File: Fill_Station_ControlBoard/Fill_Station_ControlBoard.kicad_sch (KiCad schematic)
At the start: 0 parts

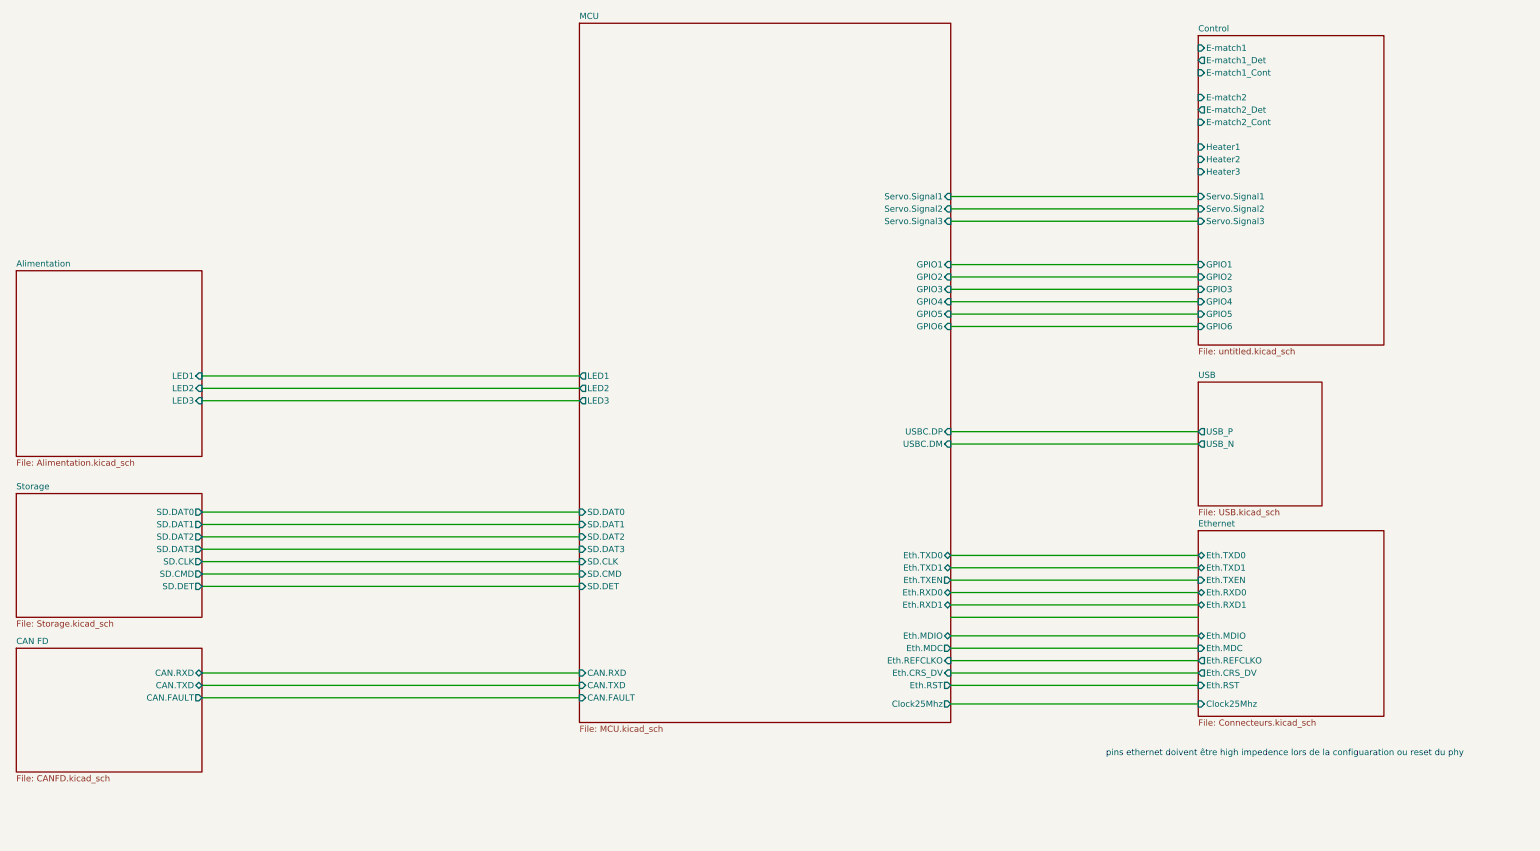
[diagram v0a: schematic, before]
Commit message: PCB fait
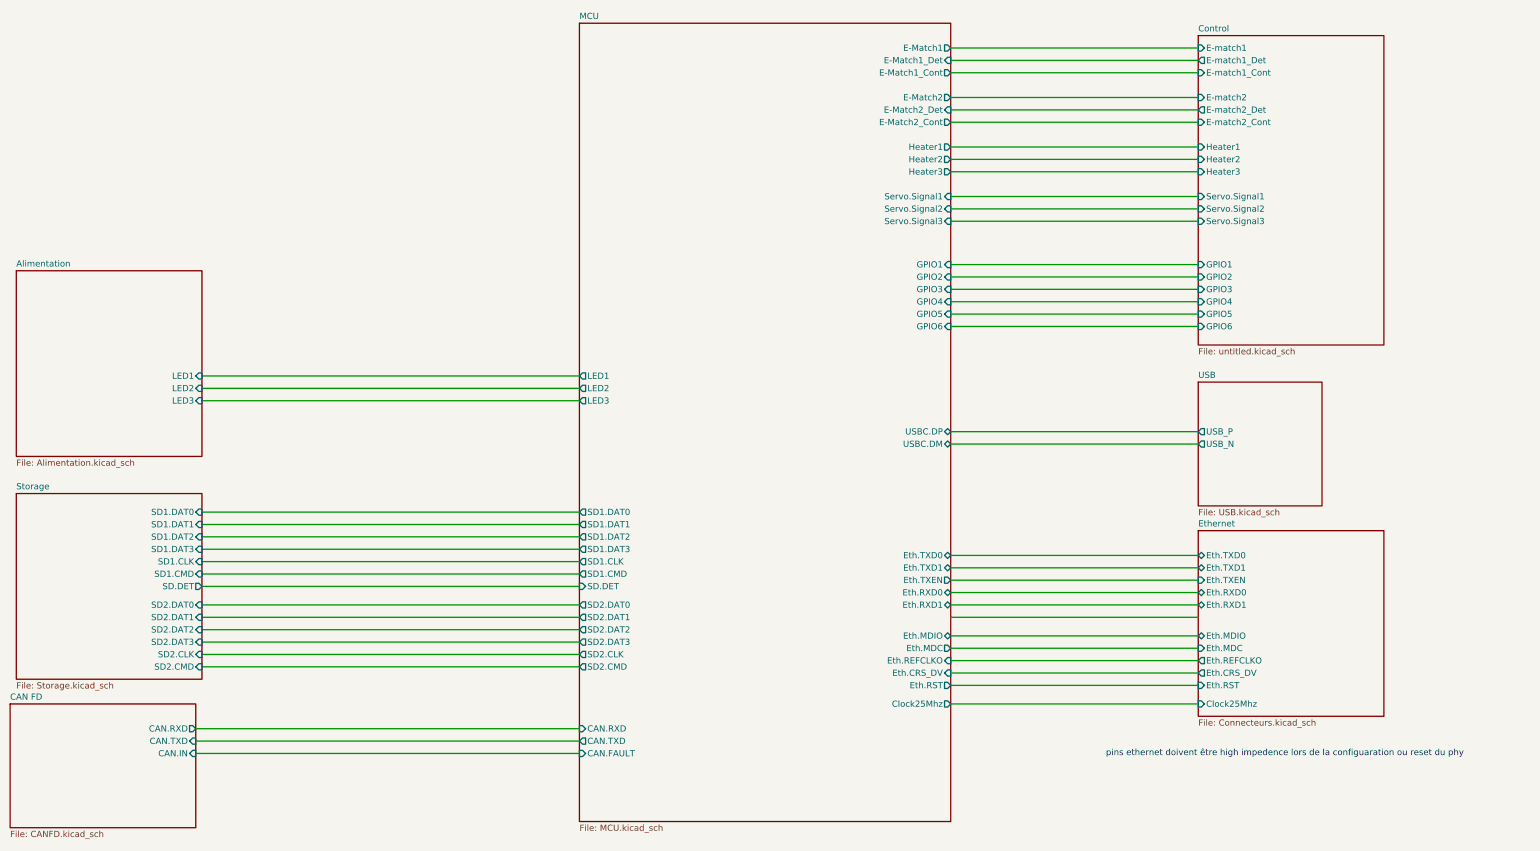
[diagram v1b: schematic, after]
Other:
- sheet CAN FD ports: added CAN.IN; removed CAN.FAULT
- sheet MCU ports: added E-Match1, E-Match1_Cont, E-Match1_Det, E-Match2, E-Match2_Cont, E-Match2_Det, Heater1, Heater2, Heater3, SD1.CLK, SD1.CMD, SD1.DAT0, SD1.DAT1, SD1.DAT2, SD1.DAT3, SD2.CLK, SD2.CMD, SD2.DAT0, SD2.DAT1, SD2.DAT2, SD2.DAT3; removed SD.CLK, SD.CMD, SD.DAT0, SD.DAT1, SD.DAT2, SD.DAT3
- sheet Storage ports: added SD1.CLK, SD1.CMD, SD1.DAT0, SD1.DAT1, SD1.DAT2, SD1.DAT3, SD2.CLK, SD2.CMD, SD2.DAT0, SD2.DAT1, SD2.DAT2, SD2.DAT3; removed SD.CLK, SD.CMD, SD.DAT0, SD.DAT1, SD.DAT2, SD.DAT3
